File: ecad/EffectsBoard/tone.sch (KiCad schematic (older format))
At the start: 5 parts, among them U1 RC4558

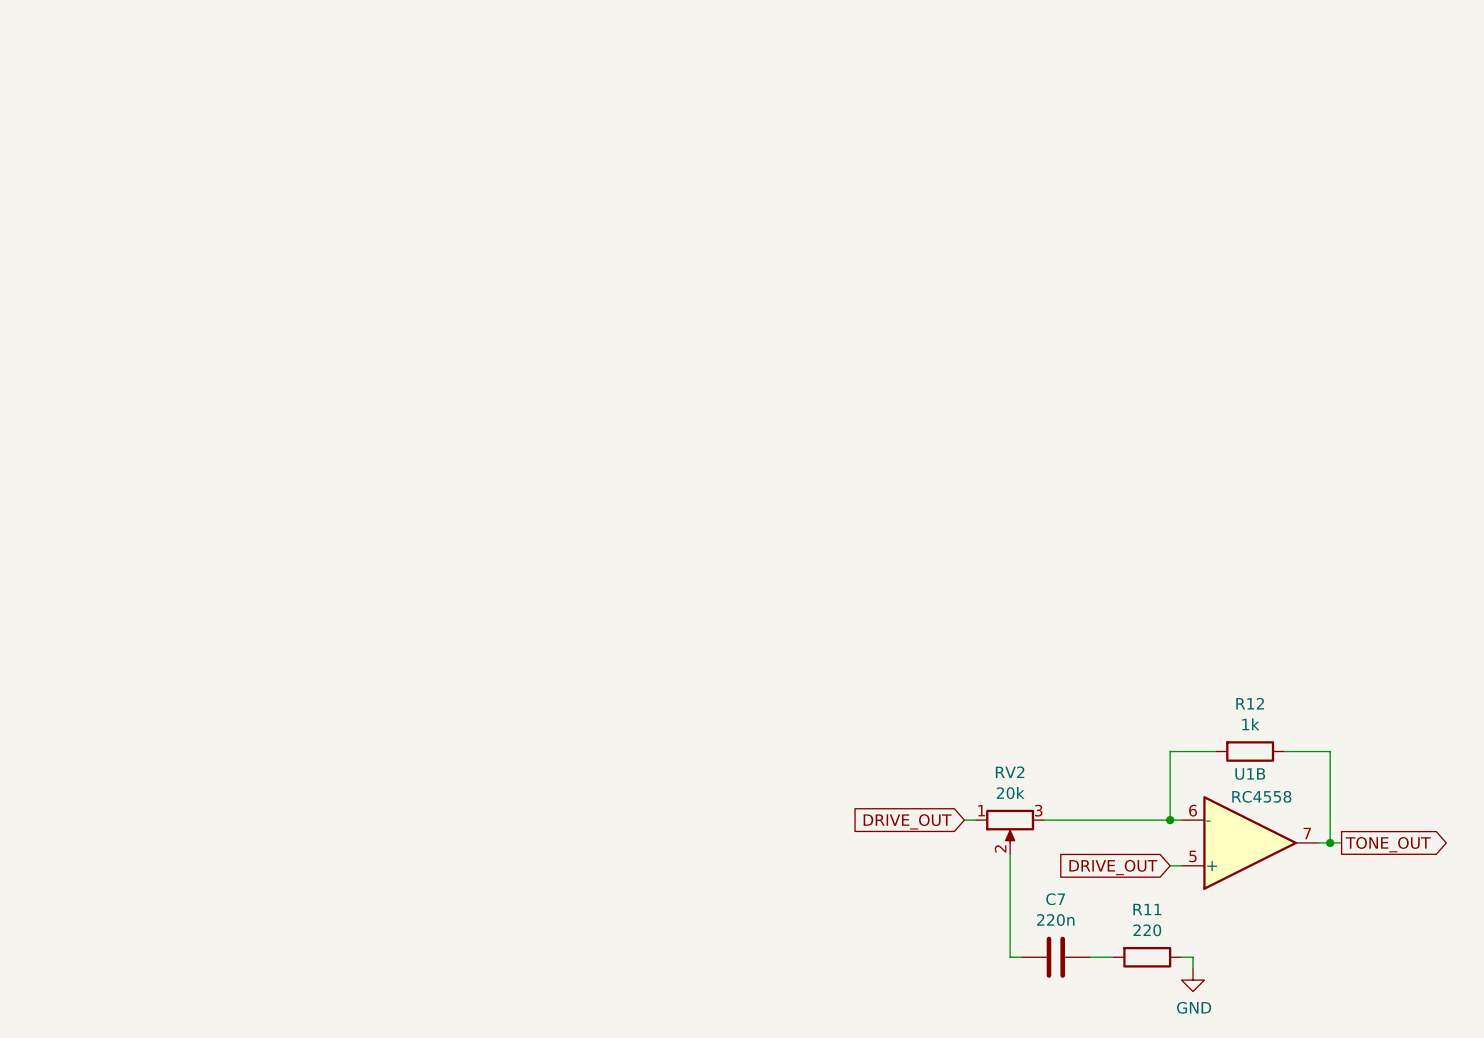
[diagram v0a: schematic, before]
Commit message: Rearrange schematics
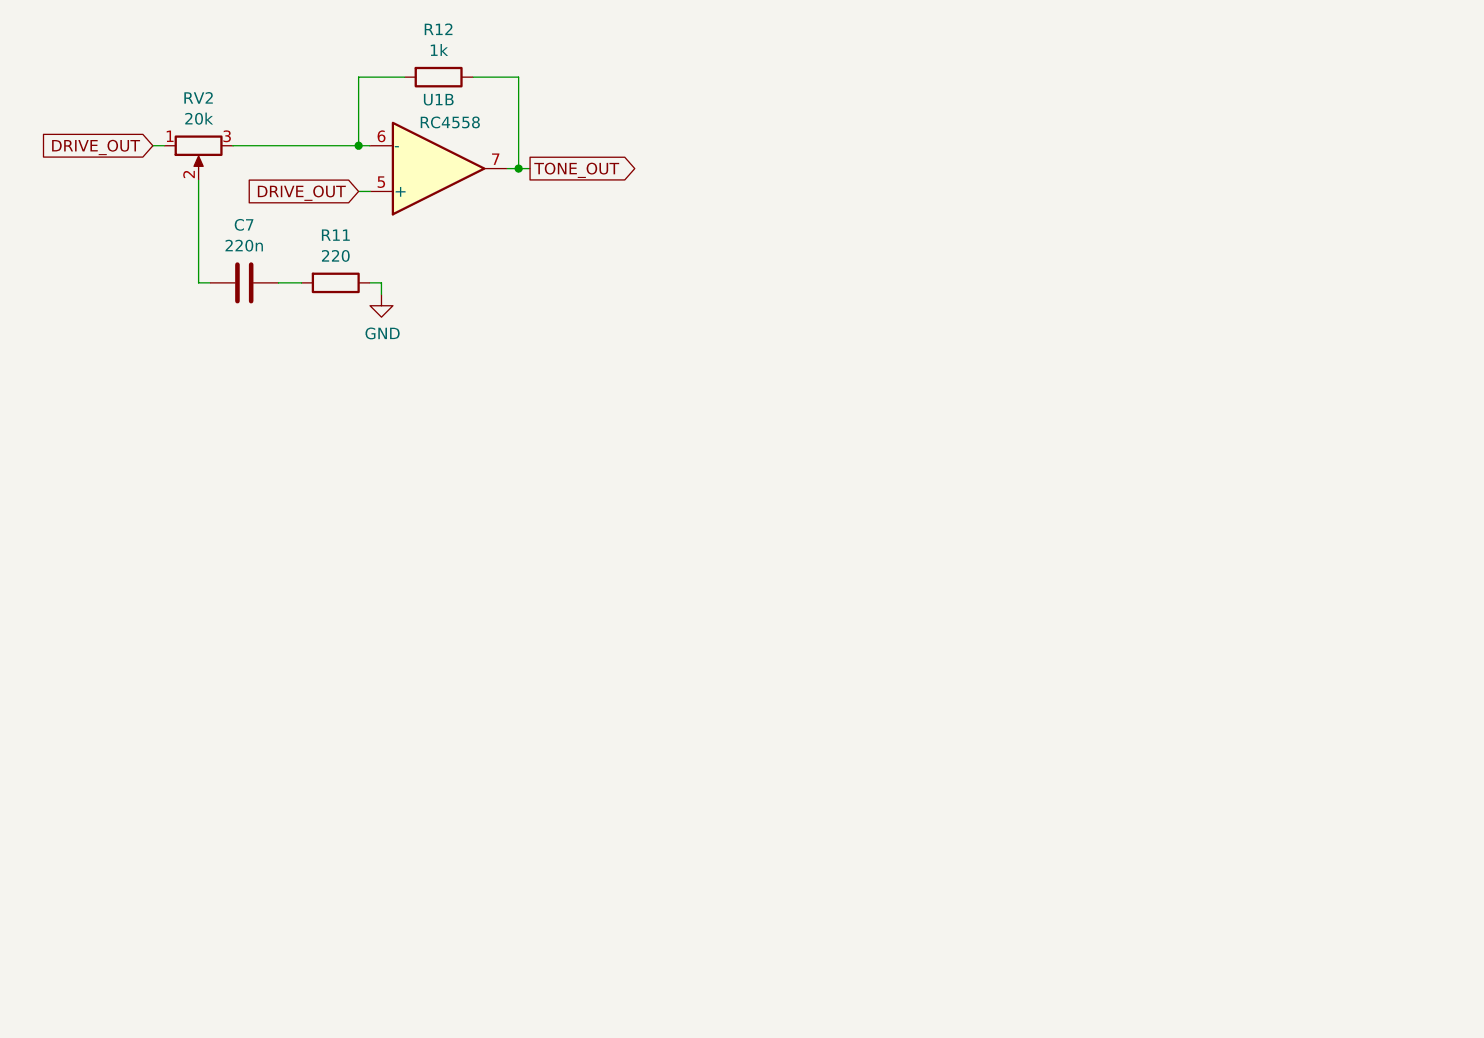
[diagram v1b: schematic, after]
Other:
- moved on the sheet: C7, R11, R12, RV2, U1B
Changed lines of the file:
@@
 L Amplifier_Operational:RC4558 U?
 U 2 1 60328176
-P 5750 4100
+P 2200 1150
 AR Path="/60328176" Ref="U?"  Part="2"
 AR Path="/60307048/60328176" Ref="U1"  Part="2"
-F 0 "U1" H 5750 3800 50  0000 C CNN
-F 1 "RC4558" H 5800 3900 50  0000 C CNN
-F 2 "" H 5750 4100 50  0001 C CNN
-F 3 "http://www.ti.com/lit/ds/symlink/rc4558.pdf" H 5750 4100 50  0001 C CNN
-	2    5750 4100
+F 0 "U1" H 2200 850 50  0000 C CNN
+F 1 "RC4558" H 2250 950 50  0000 C CNN
+F 2 "" H 2200 1150 50  0001 C CNN
+F 3 "http://www.ti.com/lit/ds/symlink/rc4558.pdf" H 2200 1150 50  0001 C CNN
+	2    2200 1150
 	1    0    0    1
 $EndComp
@@
 L Device:R R?
 U 1 1 6032817E
-P 5750 3700
+P 2200 750
 AR Path="/6032817E" Ref="R?"  Part="1"
 AR Path="/60307048/6032817E" Ref="R12"  Part="1"
-F 0 "R12" V 5543 3700 50  0000 C CNN
-F 1 "1k" V 5634 3700 50  0000 C CNN
-F 2 "" V 5680 3700 50  0001 C CNN
-F 3 "~" H 5750 3700 50  0001 C CNN
-	1    5750 3700
+F 0 "R12" V 1993 750 50  0000 C CNN
+F 1 "1k" V 2084 750 50  0000 C CNN
+F 2 "" V 2130 750 50  0001 C CNN
+F 3 "~" H 2200 750 50  0001 C CNN
+	1    2200 750
 	0    1    1    0
 $EndComp
@@
 L Device:R_POT RV?
 U 1 1 60328184
-P 4700 4000
+P 1150 1050
 AR Path="/60328184" Ref="RV?"  Part="1"
 AR Path="/60307048/60328184" Ref="RV2"  Part="1"
-F 0 "RV2" V 4493 4000 50  0000 C CNN
-F 1 "20k" V 4584 4000 50  0000 C CNN
-F 2 "" H 4700 4000 50  0001 C CNN
-F 3 "~" H 4700 4000 50  0001 C CNN
-	1    4700 4000
+F 0 "RV2" V 943 1050 50  0000 C CNN
+F 1 "20k" V 1034 1050 50  0000 C CNN
+F 2 "" H 1150 1050 50  0001 C CNN
+F 3 "~" H 1150 1050 50  0001 C CNN
+	1    1150 1050
 	0    -1   1    0
 $EndComp
@@
 L Device:C C?
 U 1 1 6032818A
-P 4900 4600
+P 1350 1650
 AR Path="/6032818A" Ref="C?"  Part="1"
 AR Path="/60307048/6032818A" Ref="C7"  Part="1"
-F 0 "C7" V 4648 4600 50  0000 C CNN
-F 1 "220n" V 4739 4600 50  0000 C CNN
-F 2 "" H 4938 4450 50  0001 C CNN
-F 3 "~" H 4900 4600 50  0001 C CNN
-	1    4900 4600
+F 0 "C7" V 1098 1650 50  0000 C CNN
+F 1 "220n" V 1189 1650 50  0000 C CNN
+F 2 "" H 1388 1500 50  0001 C CNN
+F 3 "~" H 1350 1650 50  0001 C CNN
+	1    1350 1650
 	0    1    1    0
 $EndComp
@@
 L Device:R R?
 U 1 1 60328190
-P 5300 4600
+P 1750 1650
 AR Path="/60328190" Ref="R?"  Part="1"
 AR Path="/60307048/60328190" Ref="R11"  Part="1"
-F 0 "R11" V 5093 4600 50  0000 C CNN
-F 1 "220" V 5184 4600 50  0000 C CNN
-F 2 "" V 5230 4600 50  0001 C CNN
-F 3 "~" H 5300 4600 50  0001 C CNN
-	1    5300 4600
+F 0 "R11" V 1543 1650 50  0000 C CNN
+F 1 "220" V 1634 1650 50  0000 C CNN
+F 2 "" V 1680 1650 50  0001 C CNN
+F 3 "~" H 1750 1650 50  0001 C CNN
+	1    1750 1650
 	0    1    1    0
 $EndComp
 Wire Wire Line
-	4700 4600 4750 4600
+	1150 1650 1200 1650
 Wire Wire Line
-	5050 4600 5150 4600
+	1500 1650 1600 1650
 $Comp
 L power:GND #PWR?
 U 1 1 60328199
-P 5500 4650
+P 1950 1700
 AR Path="/60328199" Ref="#PWR?"  Part="1"
 AR Path="/60307048/60328199" Ref="#PWR0118"  Part="1"
-F 0 "#PWR0118" H 5500 4400 50  0001 C CNN
-F 1 "GND" H 5505 4477 50  0000 C CNN
-F 2 "" H 5500 4650 50  0001 C CNN
-F 3 "" H 5500 4650 50  0001 C CNN
-	1    5500 4650
+F 0 "#PWR0118" H 1950 1450 50  0001 C CNN
+F 1 "GND" H 1955 1527 50  0000 C CNN
+F 2 "" H 1950 1700 50  0001 C CNN
+F 3 "" H 1950 1700 50  0001 C CNN
+	1    1950 1700
 	1    0    0    -1
 $EndComp
 Wire Wire Line
-	4850 4000 5400 4000
+	1300 1050 1850 1050
 Wire Wire Line
-	6050 4100 6100 4100
+	2500 1150 2550 1150
 Wire Wire Line
-	5400 4000 5400 3700
+	1850 1050 1850 750
 Wire Wire Line
-	5400 3700 5600 3700
+	1850 750  2050 750
 Wire Wire Line
-	6100 3700 6100 4100
+	2550 750  2550 1150
 Wire Wire Line
-	5900 3700 6100 3700
-Connection ~ 5400 4000
+	2350 750  2550 750
+Connection ~ 1850 1050
 Wire Wire Line
-	5400 4000 5450 4000
-Connection ~ 6100 4100
+	1850 1050 1900 1050
+Connection ~ 2550 1150
 Wire Wire Line
-	6100 4100 6150 4100
+	2550 1150 2600 1150
 Wire Wire Line
-	4500 4000 4550 4000
+	950  1050 1000 1050
 Wire Wire Line
-	5450 4600 5500 4600
+	1900 1650 1950 1650
 Wire Wire Line
-	5500 4600 5500 4650
-Text GLabel 4500 4000 0    50   Input ~ 0
+	1950 1650 1950 1700
+Text GLabel 950  1050 0    50   Input ~ 0
 DRIVE_OUT
-Text GLabel 5400 4200 0    50   Input ~ 0
+Text GLabel 1850 1250 0    50   Input ~ 0
 DRIVE_OUT
 Wire Wire Line
-	4700 4150 4700 4600
+	1150 1200 1150 1650
 Wire Wire Line
-	5400 4200 5450 4200
-Text GLabel 6150 4100 2    50   Output ~ 0
+	1850 1250 1900 1250
+Text GLabel 2600 1150 2    50   Output ~ 0
 TONE_OUT
 $EndSCHEMATC

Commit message: Update ecad autosave
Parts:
- C7: footprint (none) -> Capacitor_SMD:C_0805_2012Metric_Pad1.18x1.45mm_HandSolder
- R11, R12: footprint (none) -> Resistor_SMD:R_0805_2012Metric_Pad1.20x1.40mm_HandSolder
- RV2: footprint (none) -> screaming-panda:Potentiometer_Bourns_PTV09A-1_Single_Vertical
- U1: footprint (none) -> Package_SO:Texas_R-PDSO-G8_EP2.95x4.9mm_Mask2.4x3.1mm
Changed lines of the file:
@@
 F 0 "U1" H 2200 850 50  0000 C CNN
 F 1 "RC4558" H 2250 950 50  0000 C CNN
-F 2 "" H 2200 1150 50  0001 C CNN
+F 2 "Package_SO:Texas_R-PDSO-G8_EP2.95x4.9mm_Mask2.4x3.1mm" H 2200 1150 50  0001 C CNN
 F 3 "http://www.ti.com/lit/ds/symlink/rc4558.pdf" H 2200 1150 50  0001 C CNN
 	2    2200 1150
@@
 F 0 "R12" V 1993 750 50  0000 C CNN
 F 1 "1k" V 2084 750 50  0000 C CNN
-F 2 "" V 2130 750 50  0001 C CNN
+F 2 "Resistor_SMD:R_0805_2012Metric_Pad1.20x1.40mm_HandSolder" V 2130 750 50  0001 C CNN
 F 3 "~" H 2200 750 50  0001 C CNN
 	1    2200 750
@@
 F 0 "RV2" V 943 1050 50  0000 C CNN
 F 1 "20k" V 1034 1050 50  0000 C CNN
-F 2 "" H 1150 1050 50  0001 C CNN
+F 2 "screaming-panda:Potentiometer_Bourns_PTV09A-1_Single_Vertical" H 1150 1050 50  0001 C CNN
 F 3 "~" H 1150 1050 50  0001 C CNN
 	1    1150 1050
@@
 F 0 "C7" V 1098 1650 50  0000 C CNN
 F 1 "220n" V 1189 1650 50  0000 C CNN
-F 2 "" H 1388 1500 50  0001 C CNN
+F 2 "Capacitor_SMD:C_0805_2012Metric_Pad1.18x1.45mm_HandSolder" H 1388 1500 50  0001 C CNN
 F 3 "~" H 1350 1650 50  0001 C CNN
 	1    1350 1650
@@
 F 0 "R11" V 1543 1650 50  0000 C CNN
 F 1 "220" V 1634 1650 50  0000 C CNN
-F 2 "" V 1680 1650 50  0001 C CNN
+F 2 "Resistor_SMD:R_0805_2012Metric_Pad1.20x1.40mm_HandSolder" V 1680 1650 50  0001 C CNN
 F 3 "~" H 1750 1650 50  0001 C CNN
 	1    1750 1650
